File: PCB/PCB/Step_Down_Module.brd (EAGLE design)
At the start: 52 x 84.5 mm, 54 parts, among them J1 JUMPER-SMT_3_1-NC_PASTE_SILK, J2 JUMPER-SMT_3_1-NC_PASTE_SILK, J7 JUMPER-SMT_3_1-NC_PASTE_SILK, Q1 FDMC86240, Q2 FDMC86240, Q3 TPH2900ENH, U1 LTC3895_STEP_DOWN_DC-DC_CONVE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

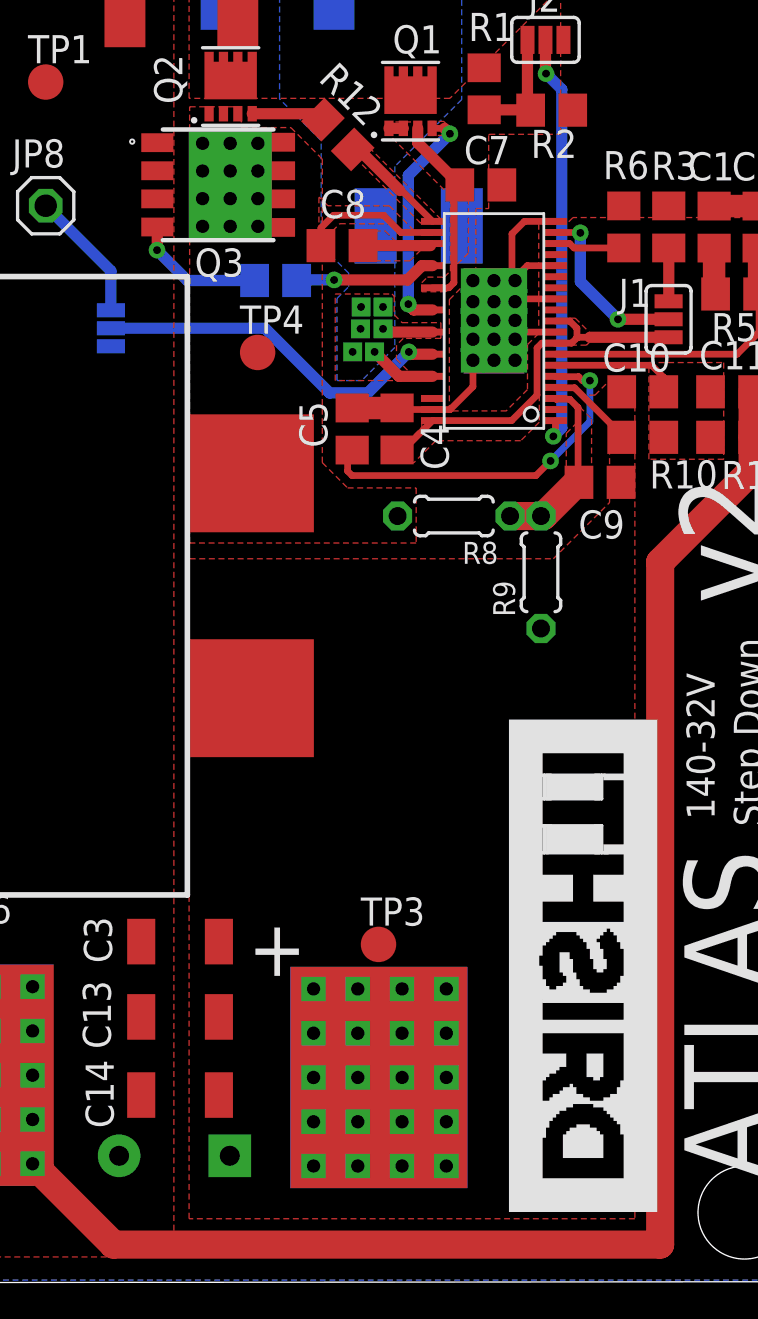
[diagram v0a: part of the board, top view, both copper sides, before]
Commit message: PCB rev2 sent for manufacture
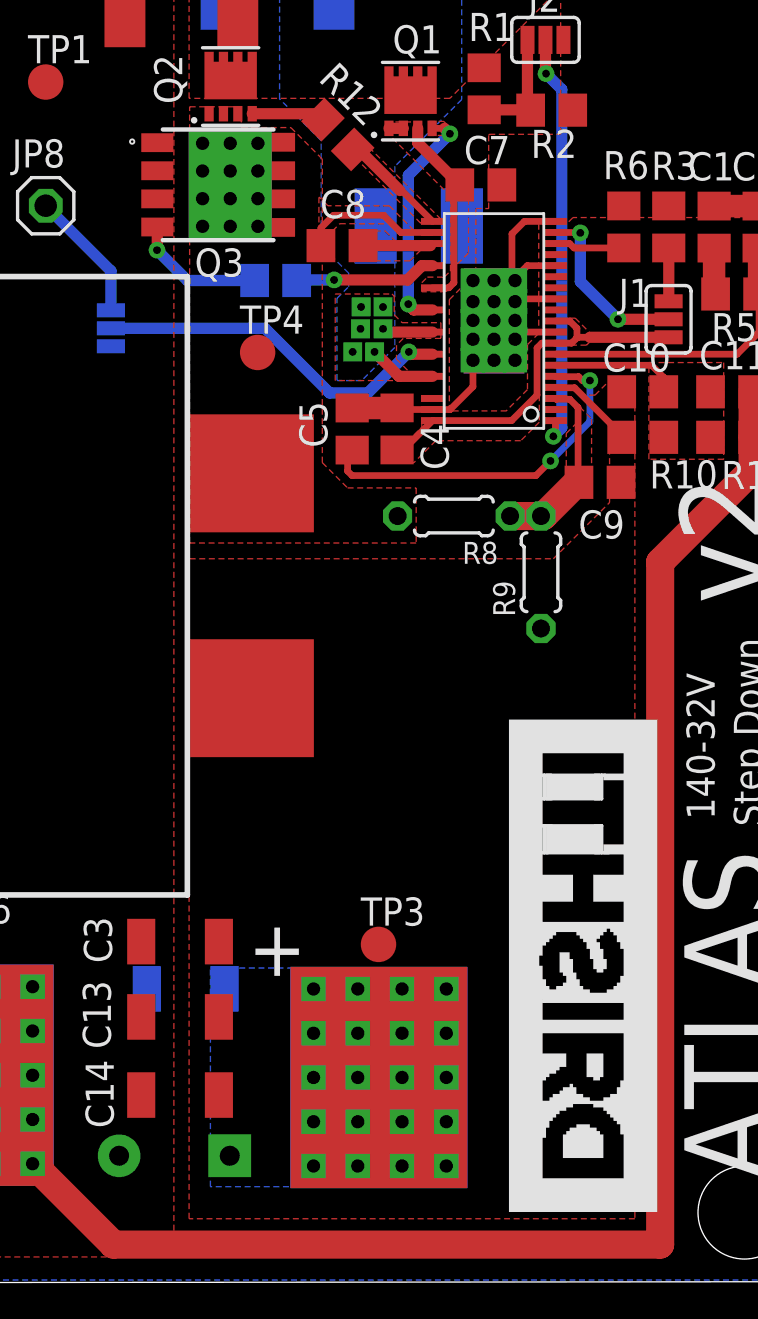
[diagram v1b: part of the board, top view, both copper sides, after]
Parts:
- added C19: 10u, SparkFun-Capacitors:1210
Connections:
- net GND: now also C19.2
- net SW: now also Q3.D1
- net VOUT: now also C19.1
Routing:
- added copper zone on layer 16, net VOUT
